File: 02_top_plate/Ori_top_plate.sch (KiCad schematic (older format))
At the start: 67 parts, among them U1 HOLE, U10 HOLE, U11 HOLE, U12 HOLE, U13 HOLE, U14 HOLE, U15 HOLE, U16 HOLE, U17 HOLE, U18 HOLE, U19 HOLE, U2 HOLE, U20 HOLE, U21 HOLE, U22 HOLE, U23 HOLE, U24 HOLE, U25 HOLE, U26 HOLE, U27 HOLE, U28 HOLE, U29 HOLE, U3 HOLE, U30 HOLE, U31 HOLE, U32 HOLE, U33 HOLE, U34 HOLE, U35 HOLE, U36 HOLE, U37 HOLE, U38 HOLE, U39 HOLE, U4 HOLE, U40 HOLE, U41 HOLE, U42 HOLE, U43 HOLE, U44 HOLE, U45 HOLE, U46 HOLE, U47 HOLE, U48 HOLE, U49 HOLE, U5 HOLE, U50 HOLE, U51 HOLE, U52 HOLE, U6 HOLE, U7 HOLE, U8 HOLE, U9 HOLE

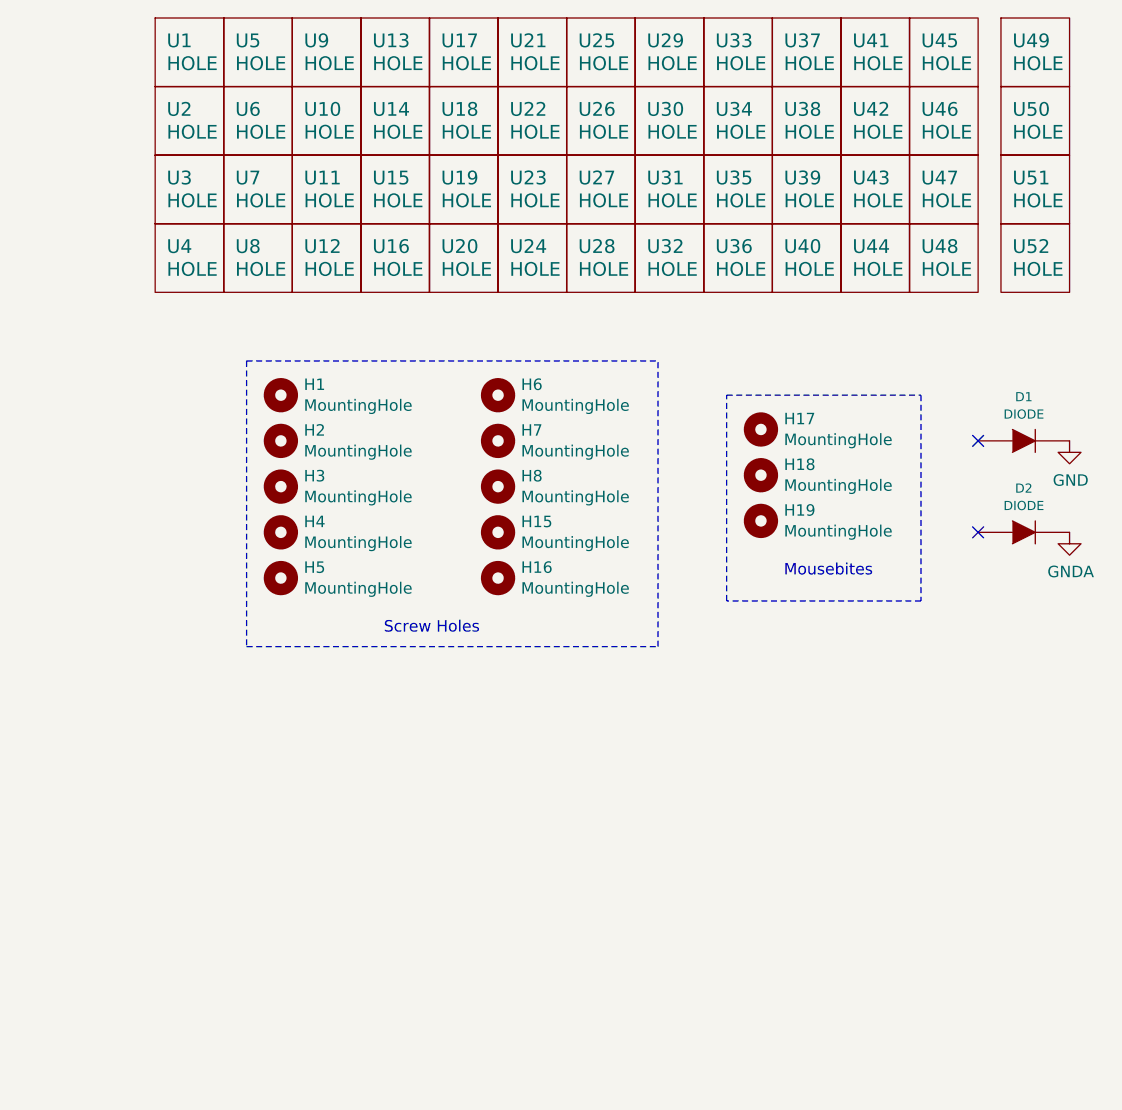
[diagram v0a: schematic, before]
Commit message: Updated firmware
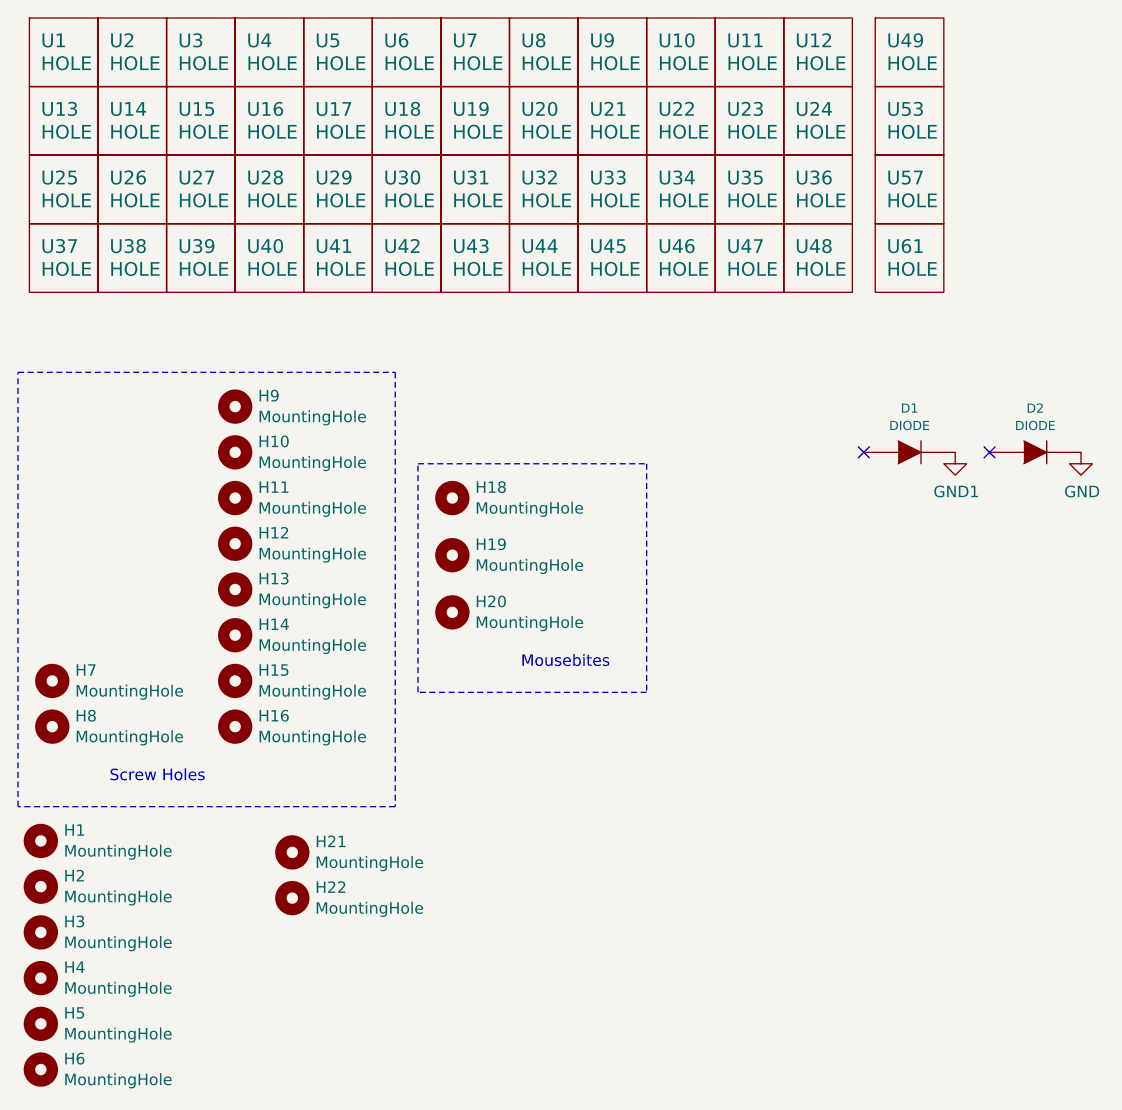
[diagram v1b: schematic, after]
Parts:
- removed H17: MountingHole, Keeb_footprints:MouseBite_IPC7351, symbol Mechanical:MountingHole
- removed U50, U51, U52: HOLE, Keebio-Parts:MX_Switch_Cutout, symbol lets_split-cache:HOLE
- added H10, H11, H12, H13, H14, H21, H22, H9: MountingHole, random-keyboard-parts:Generic-Mounthole, symbol Mechanical:MountingHole
- added H20: MountingHole, acheron_Hardware:MouseBite_IPC7351, symbol Mechanical:MountingHole
- added U53, U57, U61: HOLE, Keeb_footprints:MX100_slot, symbol lets_split-cache:HOLE
- D1, D2: footprint Diode_SMD:D_0603_1608Metric_Pad1.05x0.95mm_HandSolder -> Keeb_footprints:D_SOD-123_modified
- H1, H15, H16, H2, H3, H4, H5, H6, H7, H8: footprint random-keyboard-parts:plate_hole_4mm_tht -> random-keyboard-parts:Generic-Mounthole
- H18, H19: footprint Keeb_footprints:MouseBite_IPC7351 -> acheron_Hardware:MouseBite_IPC7351
- U1, U10, U11, U12, U13, U14, U15, U16, U17, U18, U19, U2, U20, U21, U22, U23, U24, U25, U26, U27, U28, U29, U3, U30, U31, U32, U33, U34, U35, U36, U37, U38, U39, U4, U40, U41, U42, U43, U44, U45, U46, U47, U48, U49, U5, U6, U7, U8, U9: footprint Keebio-Parts:MX_Switch_Cutout -> Keeb_footprints:MX100_slot
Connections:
- net GNDA is gone; now on net GND: D2.2 (K)
- net GND: no longer D1.2 (K)
- new net GND1: D1.2 (K)
